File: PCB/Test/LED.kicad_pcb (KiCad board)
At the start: 2 copper layers, 25 x 45 mm, 45 parts

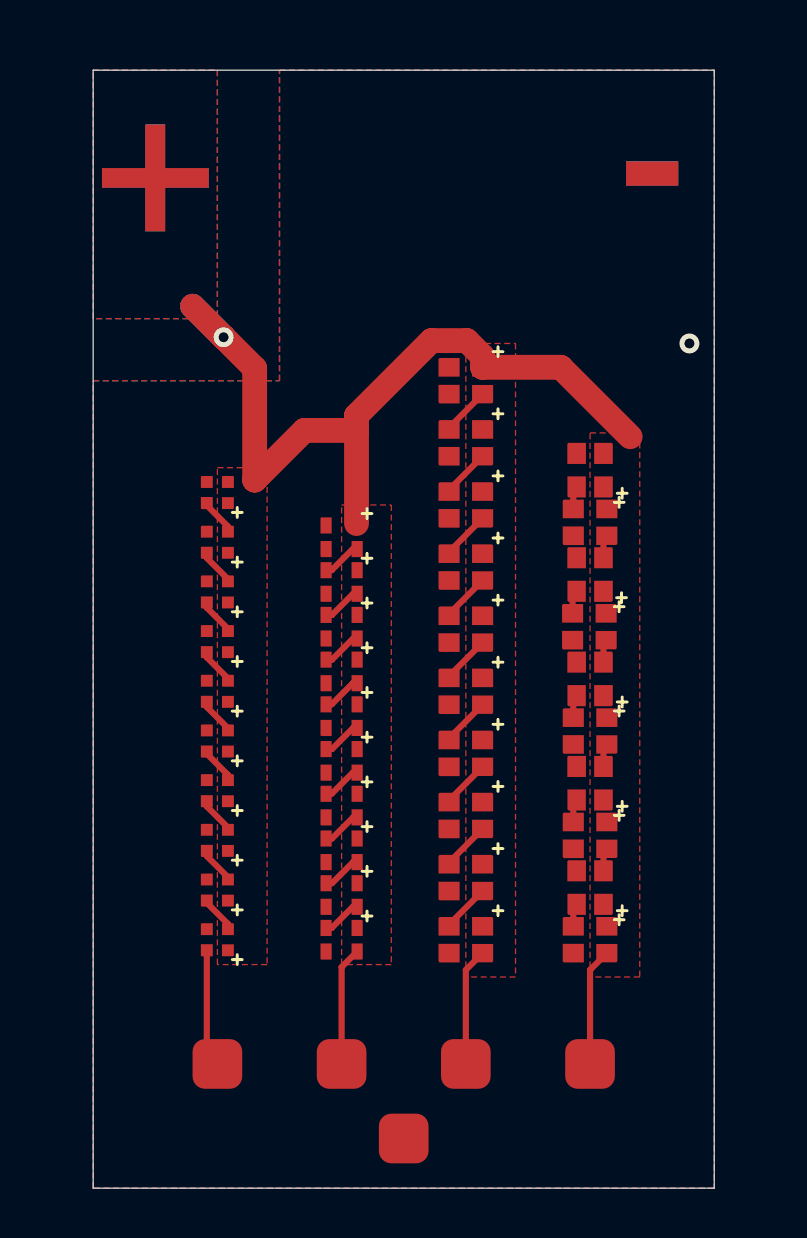
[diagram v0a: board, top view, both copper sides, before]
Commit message: Spacing
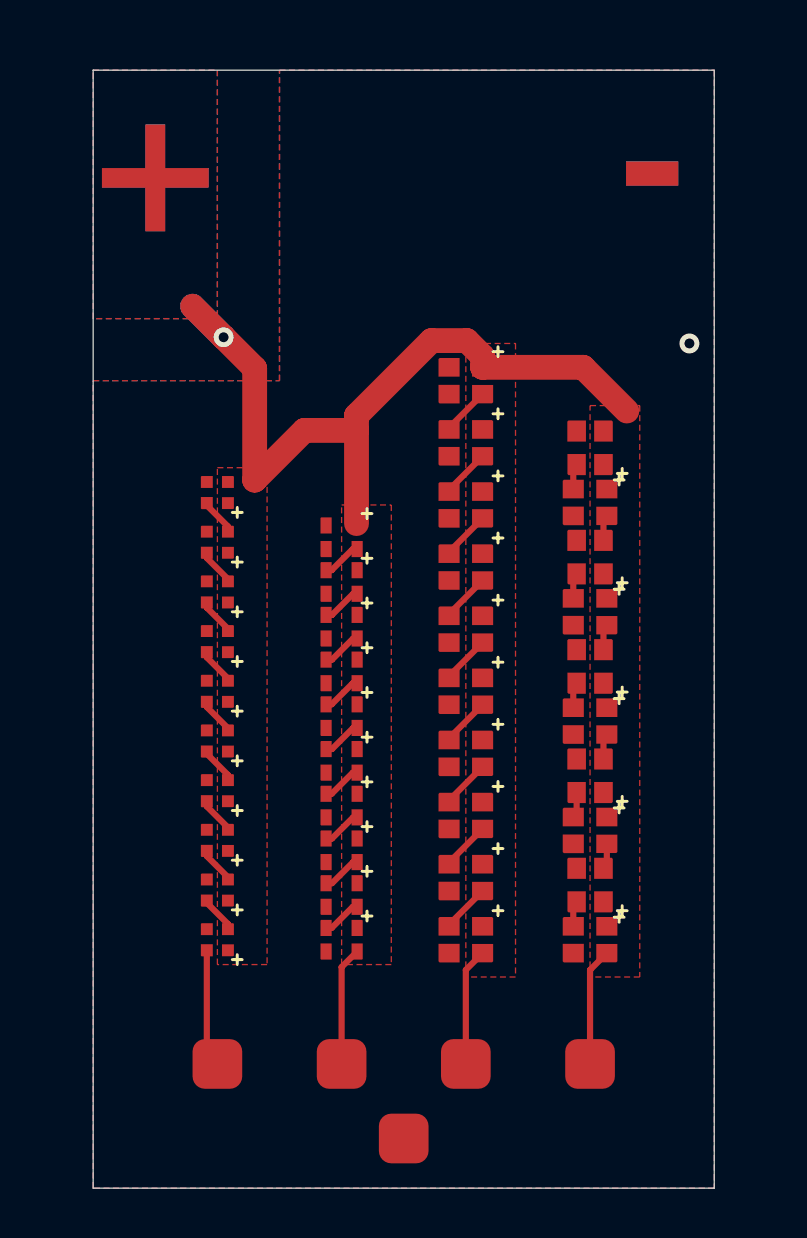
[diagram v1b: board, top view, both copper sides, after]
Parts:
- moved D40 0.90 mm to (107.5, 92.7)
- moved D39 0.80 mm to (107.5, 94.9)
- moved D38 0.70 mm to (107.5, 97.1)
- moved D37 0.60 mm to (107.5, 99.3)
- moved D36 0.50 mm to (107.5, 101.5)
- moved D35 0.40 mm to (107.5, 103.7)
- moved D34 0.30 mm to (107.5, 105.9)
- moved D33 0.20 mm to (107.5, 108.1)
- moved D32 0.10 mm to (107.5, 110.3)
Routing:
- net +3V3: track 33.2 -> 32.6 mm
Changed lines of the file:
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@@
 	(footprint "RevK:SMD2020"
 		(layer "F.Cu")
-		(at 107.5 95.7 180)
+		(at 107.5 94.9 180)
 		(descr "https://cdn-shop.adafruit.com/datasheets/WS2812B.pdf")
 		(tags "LED RGB NeoPixel")
@@
 	(footprint "RevK:SMD2020"
 		(layer "F.Cu")
-		(at 107.5 97.8 90)
+		(at 107.5 97.1 90)
 		(descr "https://cdn-shop.adafruit.com/datasheets/WS2812B.pdf")
 		(tags "LED RGB NeoPixel")
@@
 	(footprint "RevK:SMD2020"
 		(layer "F.Cu")
-		(at 107.5 104.1 180)
+		(at 107.5 103.7 180)
 		(descr "https://cdn-shop.adafruit.com/datasheets/WS2812B.pdf")
 		(tags "LED RGB NeoPixel")
@@
 	(footprint "RevK:SMD2020"
 		(layer "F.Cu")
-		(at 107.5 108.3 180)
+		(at 107.5 108.1 180)
 		(descr "https://cdn-shop.adafruit.com/datasheets/WS2812B.pdf")
 		(tags "LED RGB NeoPixel")
@@
 	(footprint "RevK:SMD2020"
 		(layer "F.Cu")
-		(at 107.5 106.2 90)
+		(at 107.5 105.9 90)
 		(descr "https://cdn-shop.adafruit.com/datasheets/WS2812B.pdf")
 		(tags "LED RGB NeoPixel")
@@
 	(footprint "RevK:SMD2020"
 		(layer "F.Cu")
-		(at 107.5 93.6 90)
+		(at 107.5 92.7 90)
 		(descr "https://cdn-shop.adafruit.com/datasheets/WS2812B.pdf")
 		(tags "LED RGB NeoPixel")
@@
 	(footprint "RevK:SMD2020"
 		(layer "F.Cu")
-		(at 107.5 102 90)
+		(at 107.5 101.5 90)
 		(descr "https://cdn-shop.adafruit.com/datasheets/WS2812B.pdf")
 		(tags "LED RGB NeoPixel")
@@
 	(footprint "RevK:SMD2020"
 		(layer "F.Cu")
-		(at 107.472659 99.902352 180)
+		(at 107.5 99.3 180)
 		(descr "https://cdn-shop.adafruit.com/datasheets/WS2812B.pdf")
 		(tags "LED RGB NeoPixel")
@@
 	(footprint "RevK:SMD2020"
 		(layer "F.Cu")
-		(at 107.5 110.4 90)
+		(at 107.5 110.3 90)
 		(descr "https://cdn-shop.adafruit.com/datasheets/WS2812B.pdf")
 		(tags "LED RGB NeoPixel")
@@
 	)
 	(segment
-		(start 98.1 92)
-		(end 98.1 95.749)
+		(start 103.175 89.46)
+		(end 107.221364 89.46)
 		(width 1)
 		(layer "F.Cu")
@@
 	)
 	(segment
-		(start 94 89.5)
-		(end 92.75 88.25)
+		(start 98.1 92)
+		(end 98.1 95.749)
 		(width 1)
 		(layer "F.Cu")
@@
 	)
 	(segment
-		(start 103.175 89.46)
-		(end 106.321364 89.46)
+		(start 94 89.5)
+		(end 92.75 88.25)
 		(width 1)
 		(layer "F.Cu")
@@
 	)
 	(segment
-		(start 106.321364 89.46)
-		(end 109.116 92.254636)
-		(width 1)
-		(layer "F.Cu")
-		(net 2)
-	)
-	(segment
 		(start 94 94)
 		(end 94 89.5)
@@
 	)
 	(segment
+		(start 107.221364 89.46)
+		(end 108.980682 91.219318)
+		(width 1)
+		(layer "F.Cu")
+		(net 2)
+	)
+	(segment
 		(start 101.116 88.384)
 		(end 98.1 91.4)
@@
 	(segment
 		(start 106.825 111.96)
-		(end 106.825 111.21)
+		(end 106.825 111.11)
 		(width 0.25)
 		(layer "F.Cu")
@@
 	)
 	(segment
-		(start 108.04 109.725)
-		(end 108.04 108.975)
+		(start 108.175 108.64)
+		(end 108.175 109.49)
 		(width 0.25)
 		(layer "F.Cu")
@@
 	)
 	(segment
-		(start 106.825 107.76)
-		(end 106.825 107.01)
+		(start 106.96 106.575)
+		(end 106.96 107.425)
 		(width 0.25)
 		(layer "F.Cu")
@@
 	)
 	(segment
-		(start 108.04 105.525)
-		(end 108.04 104.775)
+		(start 108.04 105.225)
+		(end 108.04 104.375)
 		(width 0.25)
 		(layer "F.Cu")
@@
 	)
 	(segment
-		(start 106.825 103.56)
-		(end 106.825 102.81)
+		(start 106.825 103.16)
+		(end 106.825 102.31)
 		(width 0.25)
 		(layer "F.Cu")
@@
 	)
 	(segment
-		(start 108.04 101.325)
-		(end 108.04 100.550011)
+		(start 108.04 100.825)
+		(end 108.04 99.975)
 		(width 0.25)
 		(layer "F.Cu")
@@
 	)
 	(segment
-		(start 106.797659 99.362352)
-		(end 106.797659 98.637341)
+		(start 106.825 98.76)
+		(end 106.825 97.91)
 		(width 0.25)
 		(layer "F.Cu")
@@
 	)
 	(segment
-		(start 108.04 97.125)
-		(end 108.04 96.375)
+		(start 108.04 96.425)
+		(end 108.04 95.575)
 		(width 0.25)
 		(layer "F.Cu")
@@
 	)
 	(segment
-		(start 106.825 95.16)
-		(end 106.825 94.41)
+		(start 106.825 94.36)
+		(end 106.825 93.51)
 		(width 0.25)
 		(layer "F.Cu")
@@
 		(polygon
 			(pts
-				(xy 107.5 114) (xy 107.5 92.1) (xy 109.5 92.1) (xy 109.5 114)
+				(xy 107.5 114) (xy 107.5 91) (xy 109.5 91) (xy 109.5 114)
 			)
 		)

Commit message: Tweaked design
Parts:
- D11, D12, D13, D14, D15, D16, D17, D18, D19, D20: value XL-1010RGBC-WS2812B -> XL-1615RGBC-WS2812B
- D21, D22, D23, D24, D25, D26, D27, D28, D29, D30, D31, D32, D33, D34, D35, D36, D37, D38, D39, D40: value XL-1010RGBC-WS2812B -> XL-2020RGBC-WS2812B
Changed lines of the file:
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@@
 			)
 		)
-		(property "Value" "XL-1010RGBC-WS2812B"
+		(property "Value" "XL-2020RGBC-WS2812B"
 			(at 0 2.25 0)
 			(layer "F.Fab")
@@
 			)
 		)
-		(property "Value" "XL-1010RGBC-WS2812B"
+		(property "Value" "XL-2020RGBC-WS2812B"
 			(at 0 2.25 0)
 			(layer "F.Fab")
@@
 			)
 		)
-		(property "Value" "XL-1010RGBC-WS2812B"
+		(property "Value" "XL-1615RGBC-WS2812B"
 			(at 0 2.25 0)
 			(layer "F.Fab")
@@
 			)
 		)
-		(property "Value" "XL-1010RGBC-WS2812B"
+		(property "Value" "XL-2020RGBC-WS2812B"
 			(at 0 2.25 0)
 			(layer "F.Fab")
@@
 			)
 		)
-		(property "Value" "XL-1010RGBC-WS2812B"
+		(property "Value" "XL-2020RGBC-WS2812B"
 			(at 0 2.25 0)
 			(layer "F.Fab")
@@
 			)
 		)
-		(property "Value" "XL-1010RGBC-WS2812B"
+		(property "Value" "XL-2020RGBC-WS2812B"
 			(at 0 2.25 0)
 			(layer "F.Fab")
@@
 			)
 		)
-		(property "Value" "XL-1010RGBC-WS2812B"
+		(property "Value" "XL-2020RGBC-WS2812B"
 			(at 0 2.25 0)
 			(layer "F.Fab")
@@
 			)
 		)
-		(property "Value" "XL-1010RGBC-WS2812B"
+		(property "Value" "XL-1615RGBC-WS2812B"
 			(at 0 2.25 0)
 			(layer "F.Fab")
@@
 			)
 		)
-		(property "Value" "XL-1010RGBC-WS2812B"
+		(property "Value" "XL-1615RGBC-WS2812B"
 			(at 0 2.25 0)
 			(layer "F.Fab")
@@
 			)
 		)
-		(property "Value" "XL-1010RGBC-WS2812B"
+		(property "Value" "XL-2020RGBC-WS2812B"
 			(at 0 2.25 90)
 			(layer "F.Fab")
@@
 			)
 		)
-		(property "Value" "XL-1010RGBC-WS2812B"
+		(property "Value" "XL-1615RGBC-WS2812B"
 			(at 0 2.25 0)
 			(layer "F.Fab")
@@
 			)
 		)
-		(property "Value" "XL-1010RGBC-WS2812B"
+		(property "Value" "XL-1615RGBC-WS2812B"
 			(at 0 2.25 0)
 			(layer "F.Fab")
@@
 			)
 		)
-		(property "Value" "XL-1010RGBC-WS2812B"
+		(property "Value" "XL-2020RGBC-WS2812B"
 			(at 0 2.25 0)
 			(layer "F.Fab")
@@
 			)
 		)
-		(property "Value" "XL-1010RGBC-WS2812B"
+		(property "Value" "XL-2020RGBC-WS2812B"
 			(at 0 2.25 0)
 			(layer "F.Fab")
@@
 			)
 		)
-		(property "Value" "XL-1010RGBC-WS2812B"
+		(property "Value" "XL-2020RGBC-WS2812B"
 			(at 0 2.25 0)
 			(layer "F.Fab")
@@
 			)
 		)
-		(property "Value" "XL-1010RGBC-WS2812B"
+		(property "Value" "XL-2020RGBC-WS2812B"
 			(at 0 2.25 0)
 			(layer "F.Fab")
@@
 			)
 		)
-		(property "Value" "XL-1010RGBC-WS2812B"
+		(property "Value" "XL-2020RGBC-WS2812B"
 			(at 0 2.25 0)
 			(layer "F.Fab")
@@
 			)
 		)
-		(property "Value" "XL-1010RGBC-WS2812B"
+		(property "Value" "XL-2020RGBC-WS2812B"
 			(at 0 2.25 90)
 			(layer "F.Fab")
@@
 			)
 		)
-		(property "Value" "XL-1010RGBC-WS2812B"
+		(property "Value" "XL-2020RGBC-WS2812B"
 			(at 0 2.25 0)
 			(layer "F.Fab")
@@
 			)
 		)
-		(property "Value" "XL-1010RGBC-WS2812B"
+		(property "Value" "XL-1615RGBC-WS2812B"
 			(at 0 2.25 0)
 			(layer "F.Fab")
@@
 			)
 		)
-		(property "Value" "XL-1010RGBC-WS2812B"
+		(property "Value" "XL-2020RGBC-WS2812B"
 			(at 0 2.25 90)
 			(layer "F.Fab")
@@
 			)
 		)
-		(property "Value" "XL-1010RGBC-WS2812B"
+		(property "Value" "XL-1615RGBC-WS2812B"
 			(at 0 2.25 0)
 			(layer "F.Fab")
@@
 			)
 		)
-		(property "Value" "XL-1010RGBC-WS2812B"
+		(property "Value" "XL-2020RGBC-WS2812B"
 			(at 0 2.25 90)
 			(layer "F.Fab")
@@
 			)
 		)
-		(property "Value" "XL-1010RGBC-WS2812B"
+		(property "Value" "XL-2020RGBC-WS2812B"
 			(at 0 2.25 0)
 			(layer "F.Fab")
@@
 			)
 		)
-		(property "Value" "XL-1010RGBC-WS2812B"
+		(property "Value" "XL-2020RGBC-WS2812B"
 			(at 0 2.25 0)
 			(layer "F.Fab")
@@
 			)
 		)
-		(property "Value" "XL-1010RGBC-WS2812B"
+		(property "Value" "XL-2020RGBC-WS2812B"
 			(at 0 2.25 0)
 			(layer "F.Fab")
@@
 			)
 		)
-		(property "Value" "XL-1010RGBC-WS2812B"
+		(property "Value" "XL-1615RGBC-WS2812B"
 			(at 0 2.25 0)
 			(layer "F.Fab")
@@
 			)
 		)
-		(property "Value" "XL-1010RGBC-WS2812B"
+		(property "Value" "XL-1615RGBC-WS2812B"
 			(at 0 2.25 0)
 			(layer "F.Fab")
@@
 			)
 		)
-		(property "Value" "XL-1010RGBC-WS2812B"
+		(property "Value" "XL-2020RGBC-WS2812B"
 			(at 0 2.25 90)
 			(layer "F.Fab")
@@
 			)
 		)
-		(property "Value" "XL-1010RGBC-WS2812B"
+		(property "Value" "XL-1615RGBC-WS2812B"
 			(at 0 2.25 0)
 			(layer "F.Fab")
